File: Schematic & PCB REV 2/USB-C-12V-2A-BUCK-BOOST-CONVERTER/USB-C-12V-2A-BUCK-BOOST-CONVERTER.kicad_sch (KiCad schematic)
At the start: 23 parts, among them J1 Conn_01x02_Pin, U1 TPS61089RNRR

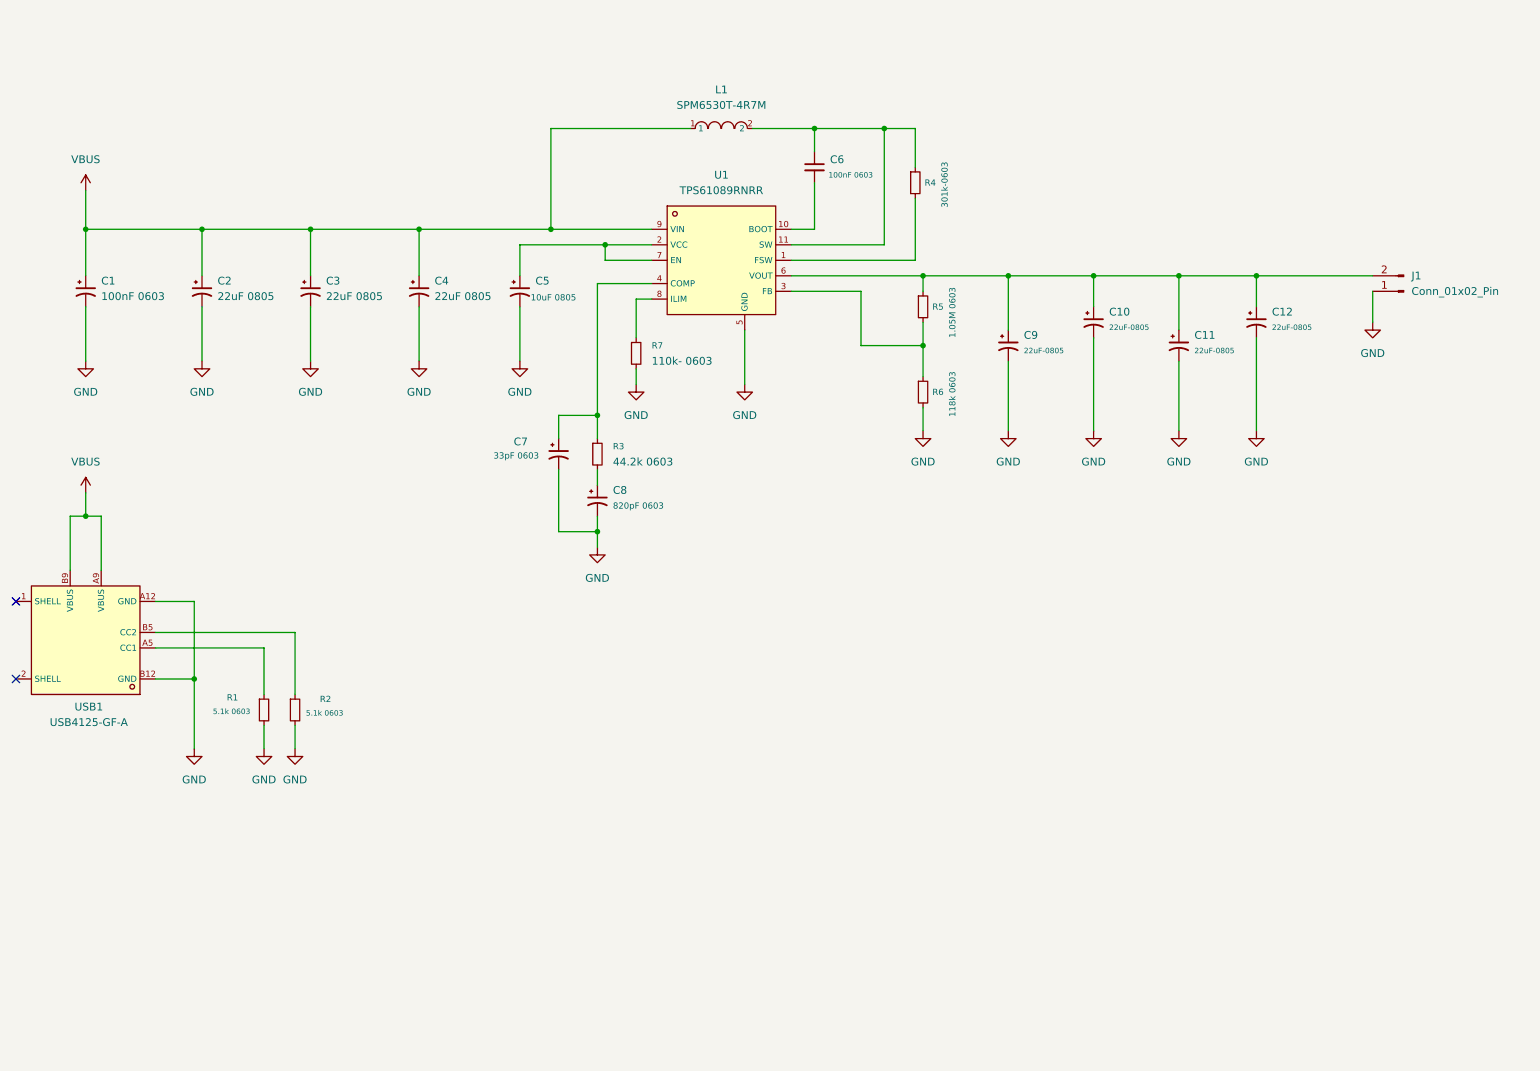
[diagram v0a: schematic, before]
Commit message: Final pcb review
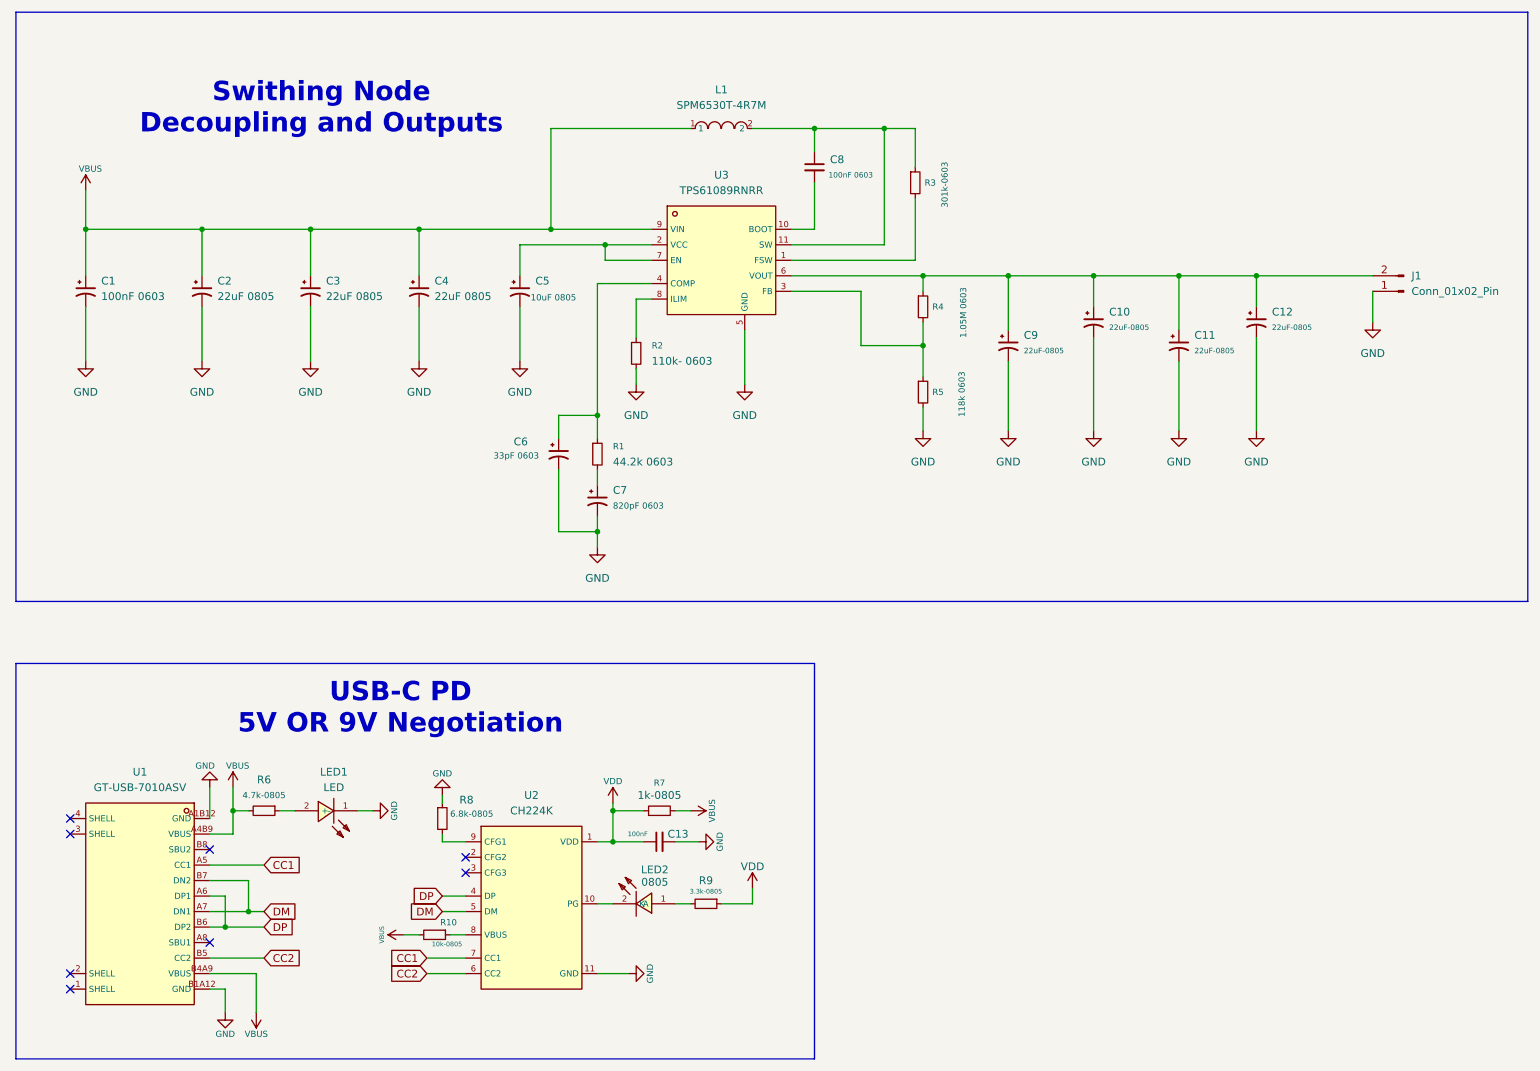
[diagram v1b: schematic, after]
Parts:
- removed R1, R2: 5.1k 0603, Resistor_SMD:R_0603_1608Metric, symbol Device:R_Small
- removed USB1: USB4125-GF-A, lcsc_footprints:C3151650_USB-C-SMD_TYPE-C-6P, symbol lcsc_imported:USB4125-GF-A
- added C13: 100nF, Capacitor_SMD:C_0603_1608Metric, symbol Device:C_Small
- added LED1: LED, lcsc_footprints:C84256_LED0805-RD, symbol lcsc_imported:LED
- added LED2: 0805, lcsc_footprints:C2297_LED0805-R-RD, symbol lcsc_imported:0805
- added R10: 10k-0805, Resistor_SMD:R_0805_2012Metric, symbol Device:R_Small
- added R6: 4.7k-0805, Resistor_SMD:R_0805_2012Metric, symbol Device:R_Small
- added R7: 1k-0805, Resistor_SMD:R_0805_2012Metric, symbol Device:R_Small
- added R8: 6.8k-0805, Resistor_SMD:R_0805_2012Metric, symbol Device:R_Small
- added R9: 3.3k-0805, Resistor_SMD:R_0805_2012Metric, symbol Device:R_Small
- added U1: GT-USB-7010ASV, lcsc_footprints:C2988369_USB-C-SMD_G-SWITCH_GT-USB-7010ASV, symbol lcsc_imported:GT-USB-7010ASV
- added U2: CH224K, lcsc_footprints:C970725_ESSOP-10_L4_9-W3_9-P1_0-LS6_0-TL-EP, symbol lcsc_imported:CH224K
- renumbered C7 to C6, C8 to C7, C6 to C8, R3 to R1, R7 to R2, R4 to R3, R5 to R4, R6 to R5, U1 to U3
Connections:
- net GND: now also C13.2, LED1.1 (-), R8.1, U1.A1B12 (GND), U1.B1A12 (GND), U2.11 (GND)
- net VBUS: now also R10.2, R6.2, R7.2, U1.A4B9 (VBUS), U1.B4A9 (VBUS)
- new net: LED2.1 (A), R9.2
- new net: LED2.2 (K), U2.10 (PG)
- new net: LED1.2 (+), R6.1
- new net: R10.1, U2.8 (VBUS)
- new net: R8.2, U2.9 (CFG1)
- new net CC1: U1.A5 (CC1), U2.7 (CC1)
- new net CC2: U1.B5 (CC2), U2.6 (CC2)
- new net DM: U1.A7 (DN1), U1.B7 (DN2), U2.5 (DM)
- new net DP: U1.A6 (DP1), U1.B6 (DP2), U2.4 (DP)
- new net VDD: C13.1, R7.1, R9.1, U2.1 (VDD)
- no-connect marks 2 -> 8
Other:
- note added: "Swithing Node Decoupling and Outputs"
- note added: "USB-C PD 5V OR 9V Negotiation"
